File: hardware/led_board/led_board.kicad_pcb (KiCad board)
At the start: 2 copper layers, 63.5 x 45.7 mm, 22 parts, among them P1 CONN_01X03, P2 CONN_01X03, P3 CONN_01X01, P4 CONN_01X01, P5 CONN_01X01, P6 CONN_01X01

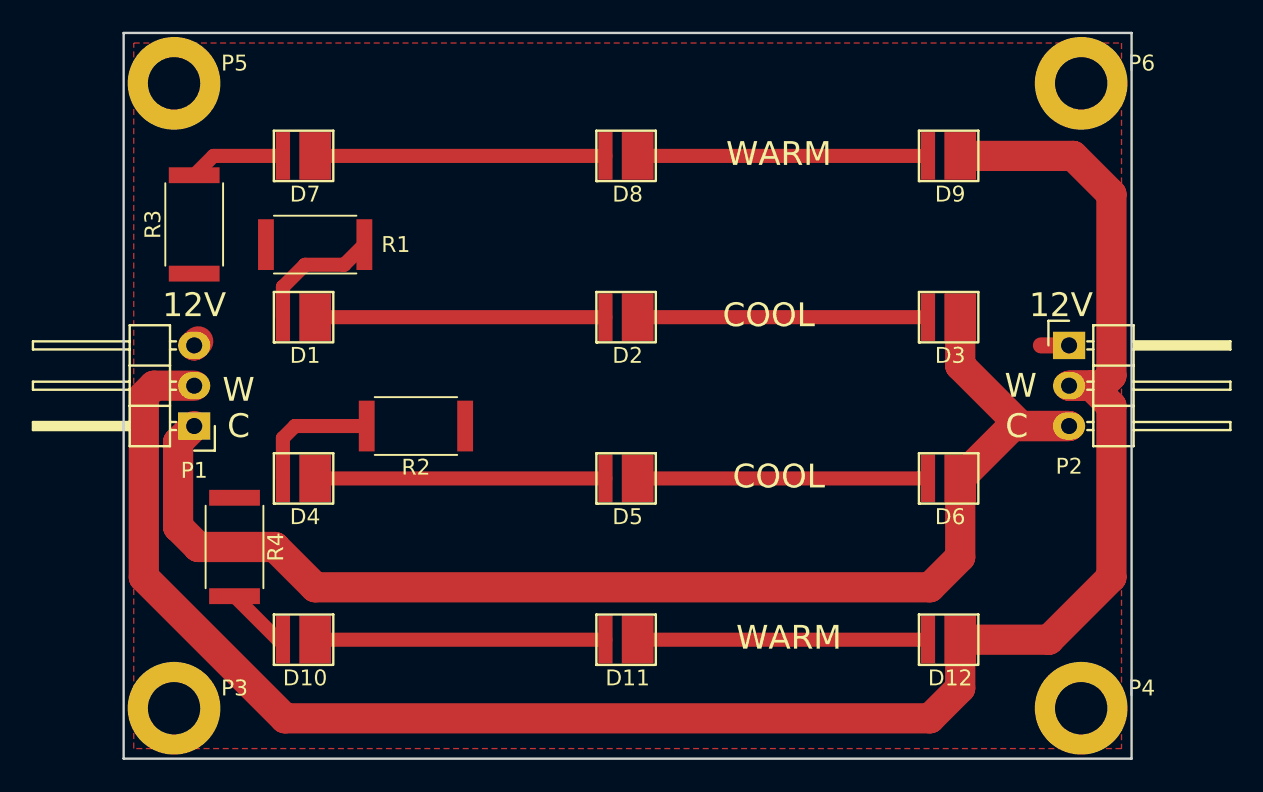
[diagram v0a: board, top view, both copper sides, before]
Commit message: Cleaned up for git import
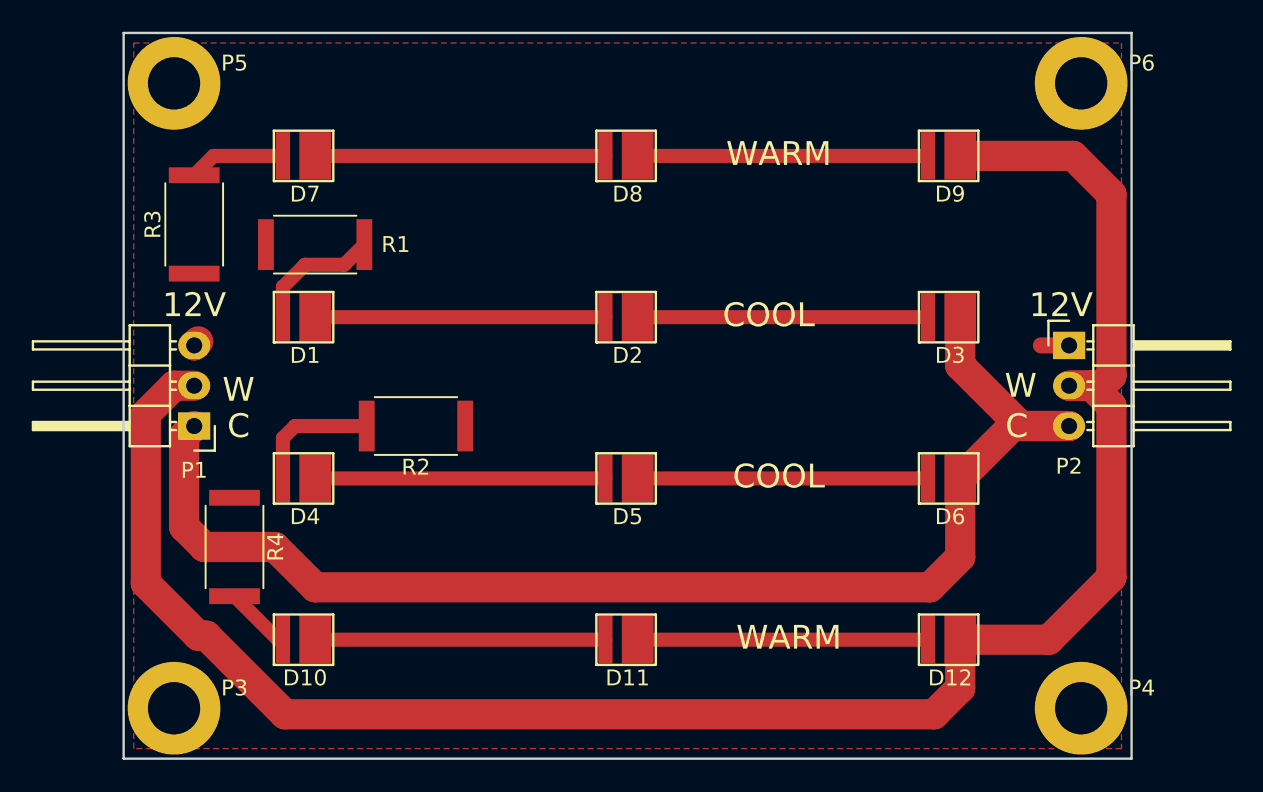
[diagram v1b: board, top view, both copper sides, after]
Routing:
- net Net-(D12-Pad1): track 123.9 -> 122.9 mm
- net Net-(D3-Pad1): track 83.1 -> 82.5 mm
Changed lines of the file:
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@@
     (thickness 1.6)
     (drawings 14)
-    (tracks 52)
+    (tracks 54)
     (zones 0)
     (modules 22)
@@
   (segment (start 160.528 94.742) (end 142.24 94.742) (width 0.889) (layer F.Cu) (net 2))
   (segment (start 180.848 94.742) (end 162.56 94.742) (width 0.889) (layer F.Cu) (net 3))
+  (segment (start 139.7 109.22) (end 135.255 109.22) (width 1.905) (layer F.Cu) (net 4))
+  (segment (start 182.88 109.855) (end 180.975 111.76) (width 1.905) (layer F.Cu) (net 4))
+  (segment (start 180.975 111.76) (end 142.24 111.76) (width 1.905) (layer F.Cu) (net 4))
+  (segment (start 142.24 111.76) (end 139.7 109.22) (width 1.905) (layer F.Cu) (net 4))
   (segment (start 182.88 104.902) (end 182.88 109.855) (width 1.905) (layer F.Cu) (net 4))
-  (segment (start 133.604002 102.615998) (end 134.62 101.6) (width 1.905) (layer F.Cu) (net 4))
-  (segment (start 133.604002 107.95) (end 133.604002 102.615998) (width 1.905) (layer F.Cu) (net 4))
-  (segment (start 134.874002 109.22) (end 133.604002 107.95) (width 1.905) (layer F.Cu) (net 4))
-  (segment (start 139.7 109.22) (end 134.874002 109.22) (width 1.905) (layer F.Cu) (net 4))
-  (segment (start 142.24 111.76) (end 139.7 109.22) (width 1.905) (layer F.Cu) (net 4))
-  (segment (start 180.975 111.76) (end 142.24 111.76) (width 1.905) (layer F.Cu) (net 4))
-  (segment (start 182.88 109.855) (end 180.975 111.76) (width 1.905) (layer F.Cu) (net 4))
+  (segment (start 133.985 107.95) (end 133.985 102.235) (width 1.905) (layer F.Cu) (net 4))
+  (segment (start 135.255 109.22) (end 133.985 107.95) (width 1.905) (layer F.Cu) (net 4))
+  (segment (start 133.985 102.235) (end 134.62 101.6) (width 1.905) (layer F.Cu) (net 4))
   (segment (start 189.738 101.6) (end 186.69 101.6) (width 1.905) (layer F.Cu) (net 4))
   (segment (start 182.88 97.79) (end 182.88 94.742) (width 1.905) (layer F.Cu) (net 4))
@@
   (segment (start 189.738 101.6) (end 186.182 101.6) (width 1.905) (layer F.Cu) (net 4))
   (segment (start 186.182 101.6) (end 182.88 104.902) (width 1.905) (layer F.Cu) (net 4))
-  (segment (start 140.208 104.902) (end 140.208 102.362) (width 0.889) (layer F.Cu) (net 5) (status 400000))
-  (segment (start 140.97 101.6) (end 145.49 101.6) (width 0.889) (layer F.Cu) (net 5) (status 800000))
+  (segment (start 140.208 104.902) (end 140.208 102.362) (width 0.889) (layer F.Cu) (net 5))
+  (segment (start 140.97 101.6) (end 145.49 101.6) (width 0.889) (layer F.Cu) (net 5))
   (segment (start 140.208 102.362) (end 140.97 101.6) (width 0.889) (layer F.Cu) (net 5))
   (segment (start 160.528 104.902) (end 142.24 104.902) (width 0.889) (layer F.Cu) (net 6))
@@
   (segment (start 142.24 84.582) (end 160.528 84.582) (width 0.889) (layer F.Cu) (net 9))
   (segment (start 162.56 84.582) (end 180.848 84.582) (width 0.889) (layer F.Cu) (net 10))
-  (segment (start 131.445 99.695) (end 131.445 111.125) (width 1.905) (layer F.Cu) (net 11))
-  (segment (start 131.445 99.695) (end 132.08 99.06) (width 1.905) (layer F.Cu) (net 11))
-  (segment (start 134.62 99.06) (end 132.08 99.06) (width 1.905) (layer F.Cu) (net 11))
-  (segment (start 180.975 120.015) (end 182.88 118.11) (width 1.905) (layer F.Cu) (net 11))
-  (segment (start 140.335 120.015) (end 180.975 120.015) (width 1.905) (layer F.Cu) (net 11))
-  (segment (start 131.445 111.125) (end 140.335 120.015) (width 1.905) (layer F.Cu) (net 11))
+  (segment (start 182.88 115.062) (end 182.88 118.11) (width 1.905) (layer F.Cu) (net 11) (status 400000))
+  (segment (start 140.335 119.761) (end 181.229 119.761) (width 1.905) (layer F.Cu) (net 11))
+  (segment (start 133.35 99.06) (end 131.572 100.838) (width 1.905) (layer F.Cu) (net 11))
+  (segment (start 131.572 100.838) (end 131.572 111.506) (width 1.905) (layer F.Cu) (net 11))
+  (segment (start 131.572 111.506) (end 134.874 114.808) (width 1.905) (layer F.Cu) (net 11))
+  (segment (start 134.874 114.808) (end 135.382 114.808) (width 1.905) (layer F.Cu) (net 11))
+  (segment (start 135.382 114.808) (end 140.335 119.761) (width 1.905) (layer F.Cu) (net 11))
+  (segment (start 133.35 99.06) (end 134.62 99.06) (width 1.905) (layer F.Cu) (net 11))
+  (segment (start 182.88 118.11) (end 181.229 119.761) (width 1.905) (layer F.Cu) (net 11))
   (segment (start 189.738 99.06) (end 191.77 99.06) (width 1.905) (layer F.Cu) (net 11))
   (segment (start 189.992 84.582) (end 182.88 84.582) (width 1.905) (layer F.Cu) (net 11))
@@
   (segment (start 192.405 98.425) (end 192.405 86.995) (width 1.905) (layer F.Cu) (net 11))
   (segment (start 191.77 99.06) (end 192.405 98.425) (width 1.905) (layer F.Cu) (net 11))
-  (segment (start 182.88 115.062) (end 182.88 118.11) (width 1.905) (layer F.Cu) (net 11))
   (segment (start 189.738 99.06) (end 191.135 99.06) (width 1.905) (layer F.Cu) (net 11))
   (segment (start 188.468 115.062) (end 182.88 115.062) (width 1.905) (layer F.Cu) (net 11))
@@
   (segment (start 192.405 100.33) (end 192.405 111.125) (width 1.905) (layer F.Cu) (net 11))
   (segment (start 191.135 99.06) (end 192.405 100.33) (width 1.905) (layer F.Cu) (net 11))
-  (segment (start 140.208 115.062) (end 139.902 115.062) (width 0.889) (layer F.Cu) (net 12) (status C00000))
-  (segment (start 139.902 115.062) (end 137.16 112.32) (width 0.889) (layer F.Cu) (net 12) (status C00000))
-  (segment (start 142.24 115.062) (end 160.528 115.062) (width 0.889) (layer F.Cu) (net 13) (status C00000))
-  (segment (start 162.56 115.062) (end 180.848 115.062) (width 0.889) (layer F.Cu) (net 14) (status C00000))
+  (segment (start 140.208 115.062) (end 139.902 115.062) (width 0.889) (layer F.Cu) (net 12))
+  (segment (start 139.902 115.062) (end 137.16 112.32) (width 0.889) (layer F.Cu) (net 12))
+  (segment (start 142.24 115.062) (end 160.528 115.062) (width 0.889) (layer F.Cu) (net 13))
+  (segment (start 162.56 115.062) (end 180.848 115.062) (width 0.889) (layer F.Cu) (net 14))
   (segment (start 134.672 96.468) (end 134.62 96.52) (width 1.905) (layer F.Cu) (net 15))
   (segment (start 134.874 96.266) (end 134.62 96.52) (width 1.905) (layer F.Cu) (net 15))
